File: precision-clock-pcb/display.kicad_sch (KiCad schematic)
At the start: 10 parts, among them U7 74HC238

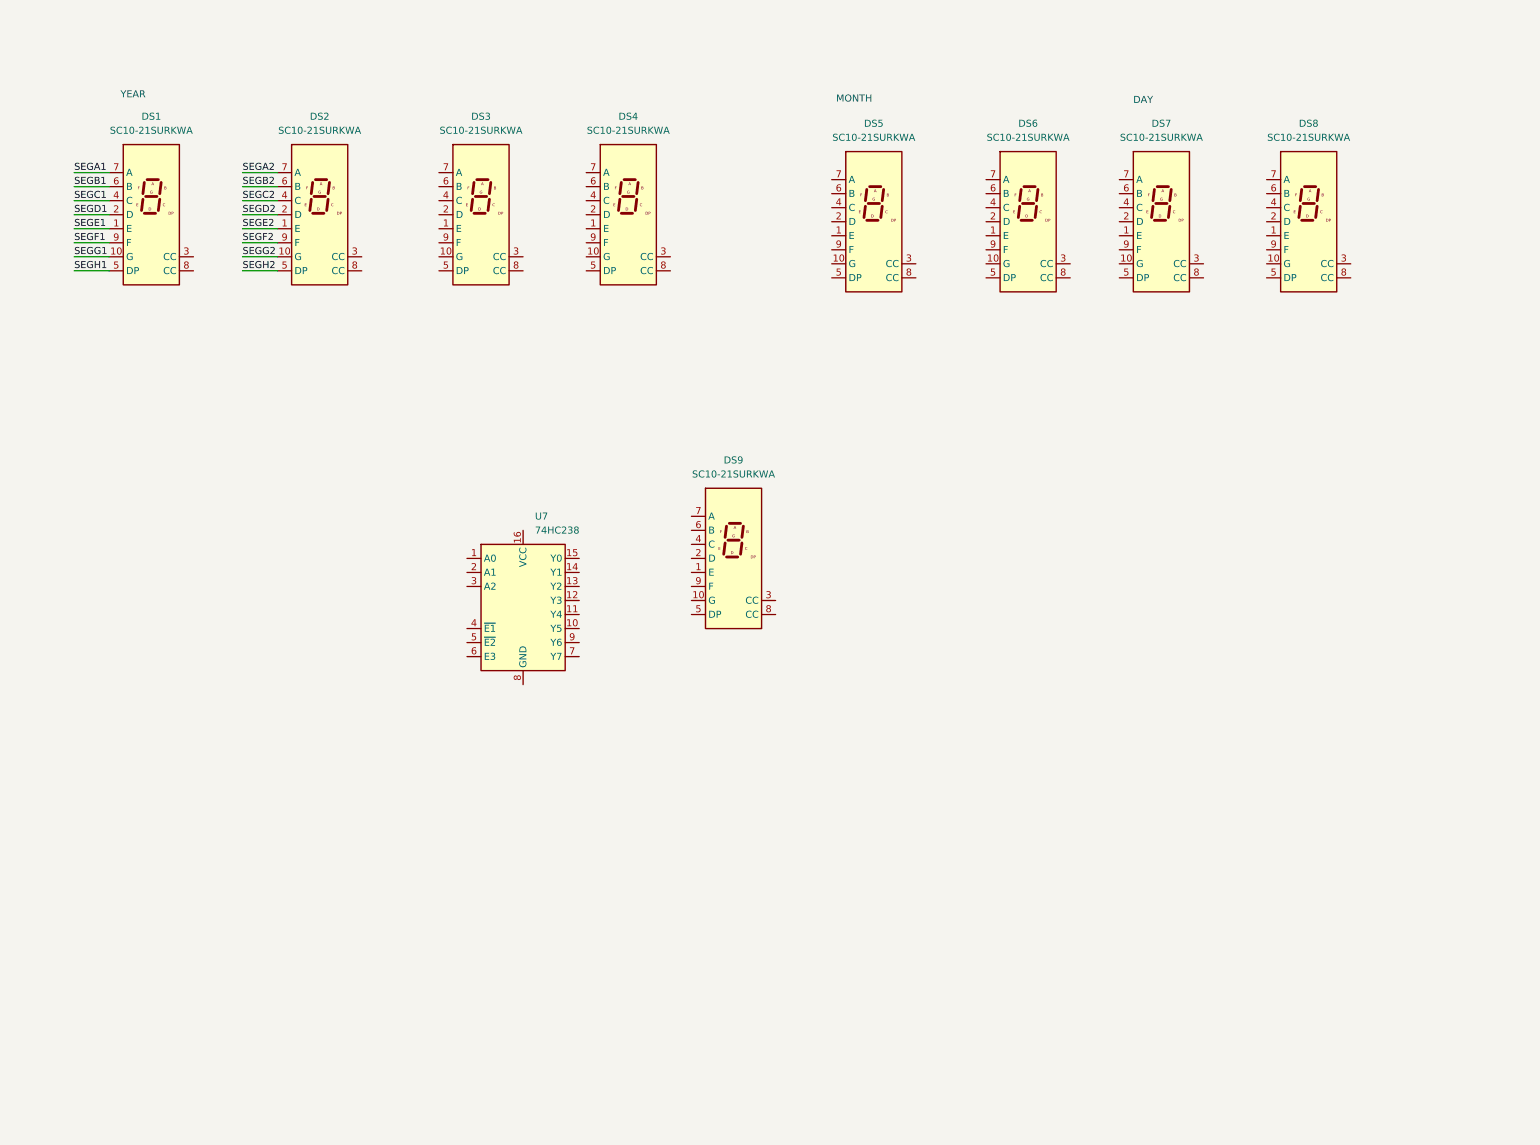
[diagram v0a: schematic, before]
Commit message: display work
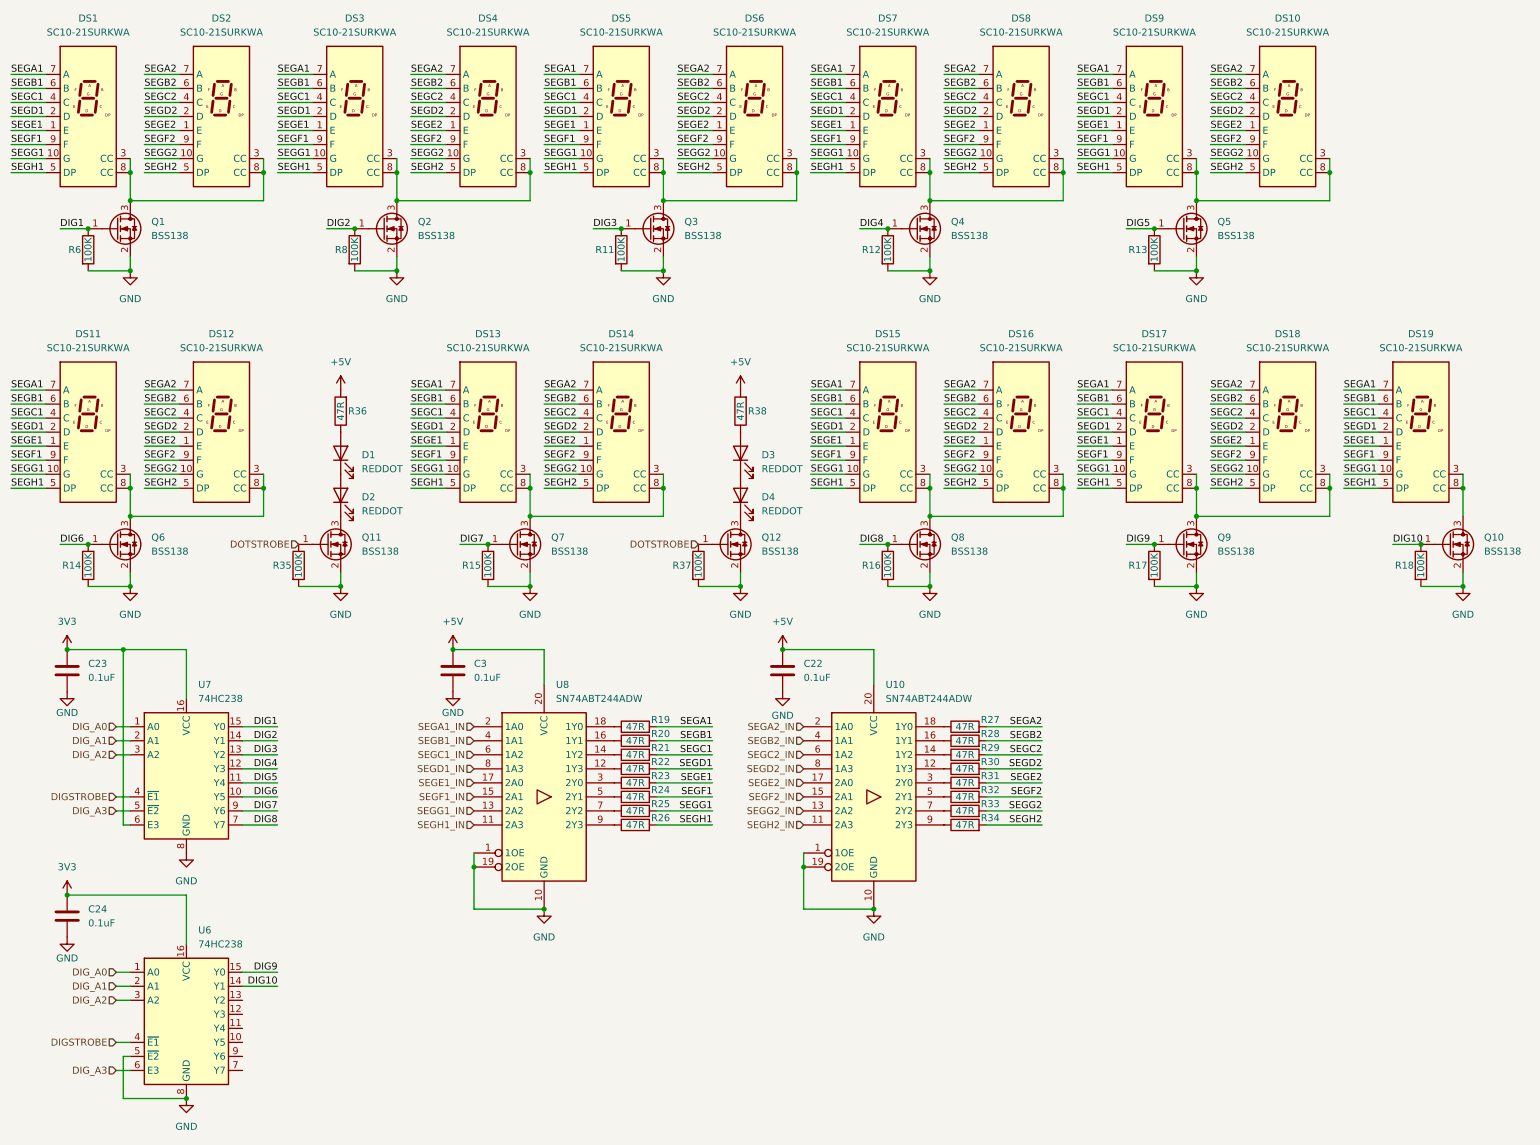
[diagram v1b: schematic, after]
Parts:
- added C22, C23, C24, C3: 0.1uF, symbol Device:C
- added D1, D2, D3, D4: REDDOT, symbol Device:LED
- added DS10, DS11, DS12, DS13, DS14, DS15, DS16, DS17, DS18, DS19: SC10-21SURKWA, Display_Custom:SC10-21SURKWA, symbol 7Segment:SC10-21SURKWA
- added Q1, Q10, Q11, Q12, Q2, Q3, Q4, Q5, Q6, Q7, Q8, Q9: BSS138, Package_TO_SOT_SMD:SOT-23, symbol Transistor_FET:BSS138
- added R11, R12, R13, R14, R15, R16, R17, R18, R35, R37, R6, R8: 100K, symbol Device:R
- added R19, R20, R21, R22, R23, R24, R25, R26, R27, R28, R29, R30, R31, R32, R33, R34, R36, R38: 47R, symbol Device:R
- added U10, U8: SN74ABT244ADW, Package_SO:SOIC-20W_7.5x12.8mm_P1.27mm, symbol 74xx:74HC244
- added U6: 74HC238, symbol 74xx:74HC238
- renumbered DS9 to DS5, DS5 to DS6, DS6 to DS7, DS7 to DS8, DS8 to DS9
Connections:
- net SEGA1: now also DS3.7 (A), DS5.7 (A), DS7.7 (A), DS9.7 (A), DS11.7 (A), DS13.7 (A), DS15.7 (A), DS17.7 (A), DS19.7 (A), R19.2
- net SEGA2: now also DS4.7 (A), DS6.7 (A), DS8.7 (A), DS10.7 (A), DS12.7 (A), DS14.7 (A), DS16.7 (A), DS18.7 (A), R27.2
- net SEGB1: now also DS3.6 (B), DS5.6 (B), DS7.6 (B), DS9.6 (B), DS11.6 (B), DS13.6 (B), DS15.6 (B), DS17.6 (B), DS19.6 (B), R20.2
- net SEGB2: now also DS4.6 (B), DS6.6 (B), DS8.6 (B), DS10.6 (B), DS12.6 (B), DS14.6 (B), DS16.6 (B), DS18.6 (B), R28.2
- net SEGC1: now also DS3.4 (C), DS5.4 (C), DS7.4 (C), DS9.4 (C), DS11.4 (C), DS13.4 (C), DS15.4 (C), DS17.4 (C), DS19.4 (C), R21.2
- net SEGC2: now also DS4.4 (C), DS6.4 (C), DS8.4 (C), DS10.4 (C), DS12.4 (C), DS14.4 (C), DS16.4 (C), DS18.4 (C), R29.2
- net SEGD1: now also DS3.2 (D), DS5.2 (D), DS7.2 (D), DS9.2 (D), DS11.2 (D), DS13.2 (D), DS15.2 (D), DS17.2 (D), DS19.2 (D), R22.2
- net SEGD2: now also DS4.2 (D), DS6.2 (D), DS8.2 (D), DS10.2 (D), DS12.2 (D), DS14.2 (D), DS16.2 (D), DS18.2 (D), R30.2
- net SEGE1: now also DS3.1 (E), DS5.1 (E), DS7.1 (E), DS9.1 (E), DS11.1 (E), DS13.1 (E), DS15.1 (E), DS17.1 (E), DS19.1 (E), R23.2
- net SEGE2: now also DS4.1 (E), DS6.1 (E), DS8.1 (E), DS10.1 (E), DS12.1 (E), DS14.1 (E), DS16.1 (E), DS18.1 (E), R31.2
- net SEGF1: now also DS3.9 (F), DS5.9 (F), DS7.9 (F), DS9.9 (F), DS11.9 (F), DS13.9 (F), DS15.9 (F), DS17.9 (F), DS19.9 (F), R24.2
- net SEGF2: now also DS4.9 (F), DS6.9 (F), DS8.9 (F), DS10.9 (F), DS12.9 (F), DS14.9 (F), DS16.9 (F), DS18.9 (F), R32.2
- net SEGG1: now also DS3.10 (G), DS5.10 (G), DS7.10 (G), DS9.10 (G), DS11.10 (G), DS13.10 (G), DS15.10 (G), DS17.10 (G), DS19.10 (G), R25.2
- net SEGG2: now also DS4.10 (G), DS6.10 (G), DS8.10 (G), DS10.10 (G), DS12.10 (G), DS14.10 (G), DS16.10 (G), DS18.10 (G), R33.2
- net SEGH1: now also DS3.5 (DP), DS5.5 (DP), DS7.5 (DP), DS9.5 (DP), DS11.5 (DP), DS13.5 (DP), DS15.5 (DP), DS17.5 (DP), DS19.5 (DP), R26.2
- net SEGH2: now also DS4.5 (DP), DS6.5 (DP), DS8.5 (DP), DS10.5 (DP), DS12.5 (DP), DS14.5 (DP), DS16.5 (DP), DS18.5 (DP), R34.2
- net at DS3.3 (CC): now also DS3.8 (CC), DS4.3 (CC), DS4.8 (CC), Q2.3 (D)
- net at DS9.3 (CC): now also DS9.8 (CC), DS10.3 (CC), DS10.8 (CC), Q5.3 (D)
- net DIG_A0: now reaches U7.1 (A0)
- net DIG_A0: now also U6.1 (A0)
- net DIG6: now reaches U7.10 (Y5)
- net DIG6: now also Q6.1 (G), R14.1
- net DIG5: now reaches U7.11 (Y4)
- net DIG5: now also Q5.1 (G), R13.1
- net DIG4: now reaches U7.12 (Y3)
- net DIG4: now also Q4.1 (G), R12.1
- net DIG3: now reaches U7.13 (Y2)
- net DIG3: now also Q3.1 (G), R11.1
- net DIG2: now reaches U7.14 (Y1)
- net DIG2: now also Q2.1 (G), R8.1
- net DIG1: now reaches U7.15 (Y0)
- net DIG1: now also Q1.1 (G), R6.1
- net 3V3: now reaches U7.16 (VCC)
- net 3V3: now also U7.6 (E3), C23.1, C24.1, U6.16 (VCC)
- net DIG_A1: now reaches U7.2 (A1)
- net DIG_A1: now also U6.2 (A1)
- net DIG_A2: now reaches U7.3 (A2)
- net DIG_A2: now also U6.3 (A2)
- net DIGSTROBE: now reaches U7.4 (~{E1})
- net DIGSTROBE: now also U6.4 (~{E1})
- net DIG_A3: now reaches U7.5 (~{E2})
- net DIG_A3: now also U6.6 (E3)
- net DIG8: now reaches U7.7 (Y7)
- net DIG8: now also Q8.1 (G), R16.1
- net GND: now reaches U7.8 (GND)
- net GND: now also C22.2, C23.2, C24.2, C3.2, Q1.2 (S), Q10.2 (S), Q11.2 (S), Q12.2 (S), Q2.2 (S), Q3.2 (S), Q4.2 (S), Q5.2 (S), Q6.2 (S), Q7.2 (S), Q8.2 (S), Q9.2 (S), R11.2, R12.2, R13.2, R14.2, R15.2, R16.2, R17.2, R18.2, R35.2, R37.2, R6.2, R8.2, U10.1 (1OE), U10.10 (GND), U10.19 (2OE), U6.5 (~{E2}), U6.8 (GND), U8.1 (1OE), U8.10 (GND), U8.19 (2OE)
- net DIG7: now reaches U7.9 (Y6)
- net DIG7: now also Q7.1 (G), R15.1
- net at DS8.3 (CC): now also DS7.3 (CC), DS7.8 (CC), DS8.8 (CC), Q4.3 (D)
- net at DS6.3 (CC): now also DS5.3 (CC), DS5.8 (CC), DS6.8 (CC), Q3.3 (D)
- net at DS2.3 (CC): now also DS1.3 (CC), DS1.8 (CC), DS2.8 (CC), Q1.3 (D)
- new net: DS11.3 (CC), DS11.8 (CC), DS12.3 (CC), DS12.8 (CC), Q6.3 (D)
- new net: D1.2 (A), R36.1
- new net: R21.1, U8.14 (1Y2)
- new net: D2.1 (K), Q11.3 (D)
- new net: R22.1, U8.12 (1Y3)
- new net: R20.1, U8.16 (1Y1)
- new net: R19.1, U8.18 (1Y0)
- new net: R23.1, U8.3 (2Y0)
- new net: R24.1, U8.5 (2Y1)
- new net: R25.1, U8.7 (2Y2)
- new net: R26.1, U8.9 (2Y3)
- new net: DS15.3 (CC), DS15.8 (CC), DS16.3 (CC), DS16.8 (CC), Q8.3 (D)
- new net: R34.1, U10.9 (2Y3)
- new net: R29.1, U10.14 (1Y2)
- new net: R32.1, U10.5 (2Y1)
- new net: D3.1 (K), D4.2 (A)
- new net: D3.2 (A), R38.1
- new net: R30.1, U10.12 (1Y3)
- new net: R28.1, U10.16 (1Y1)
- new net: R27.1, U10.18 (1Y0)
- new net: R31.1, U10.3 (2Y0)
- new net: R33.1, U10.7 (2Y2)
- new net: DS13.3 (CC), DS13.8 (CC), DS14.3 (CC), DS14.8 (CC), Q7.3 (D)
- new net: DS17.3 (CC), DS17.8 (CC), DS18.3 (CC), DS18.8 (CC), Q9.3 (D)
- new net: D1.1 (K), D2.2 (A)
- new net: D4.1 (K), Q12.3 (D)
- new net: DS19.3 (CC), DS19.8 (CC), Q10.3 (D)
- new net +5V: C22.1, C3.1, R36.2, R38.2, U10.20 (VCC), U8.20 (VCC)
- new net DIG10: Q10.1 (G), R18.1, U6.14 (Y1)
- new net DIG9: Q9.1 (G), R17.1, U6.15 (Y0)
- new net DOTSTROBE: Q11.1 (G), Q12.1 (G), R35.1, R37.1
- new net SEGA1_IN: U8.2 (1A0)
- new net SEGA2_IN: U10.2 (1A0)
- new net SEGB1_IN: U8.4 (1A1)
- new net SEGB2_IN: U10.4 (1A1)
- new net SEGC1_IN: U8.6 (1A2)
- new net SEGC2_IN: U10.6 (1A2)
- new net SEGD1_IN: U8.8 (1A3)
- new net SEGD2_IN: U10.8 (1A3)
- new net SEGE1_IN: U8.17 (2A0)
- new net SEGE2_IN: U10.17 (2A0)
- new net SEGF1_IN: U8.15 (2A1)
- new net SEGF2_IN: U10.15 (2A1)
- new net SEGG1_IN: U8.13 (2A2)
- new net SEGG2_IN: U10.13 (2A2)
- new net SEGH1_IN: U8.11 (2A3)
- new net SEGH2_IN: U10.11 (2A3)
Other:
- note removed: "DAY"
- note removed: "MONTH"
- note removed: "YEAR"
- moved on the sheet: DS1, DS2, DS3, DS4, DS5, DS6, DS7, DS8, DS9, U7
